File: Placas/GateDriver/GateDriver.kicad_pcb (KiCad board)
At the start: 2 copper layers, 71 x 41 mm, 30 parts, among them J1 Conn_02x04_Odd_Even, J2 Conn_02x04_Odd_Even, Q1 BD135, Q2 BD136, U1 74HC14, U2 LM7815_TO220, U3 HCPL-3120

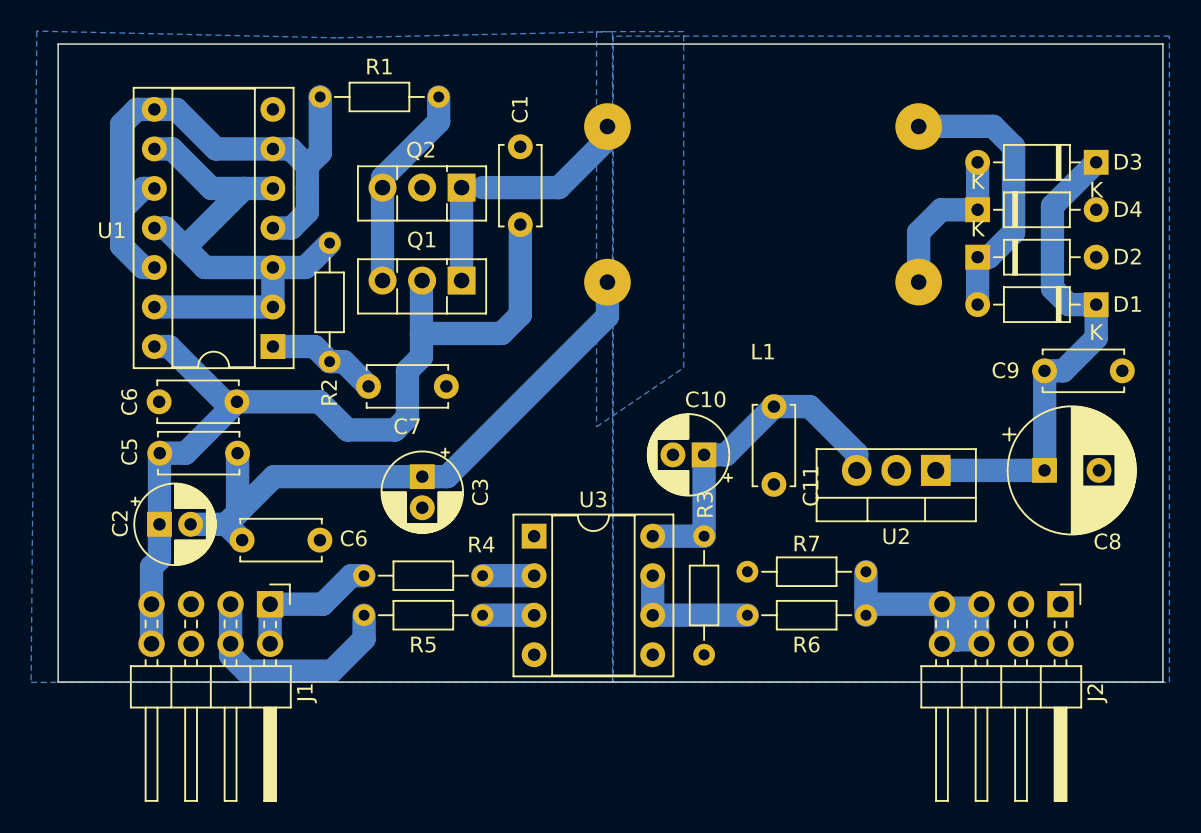
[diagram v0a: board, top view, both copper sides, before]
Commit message: Working
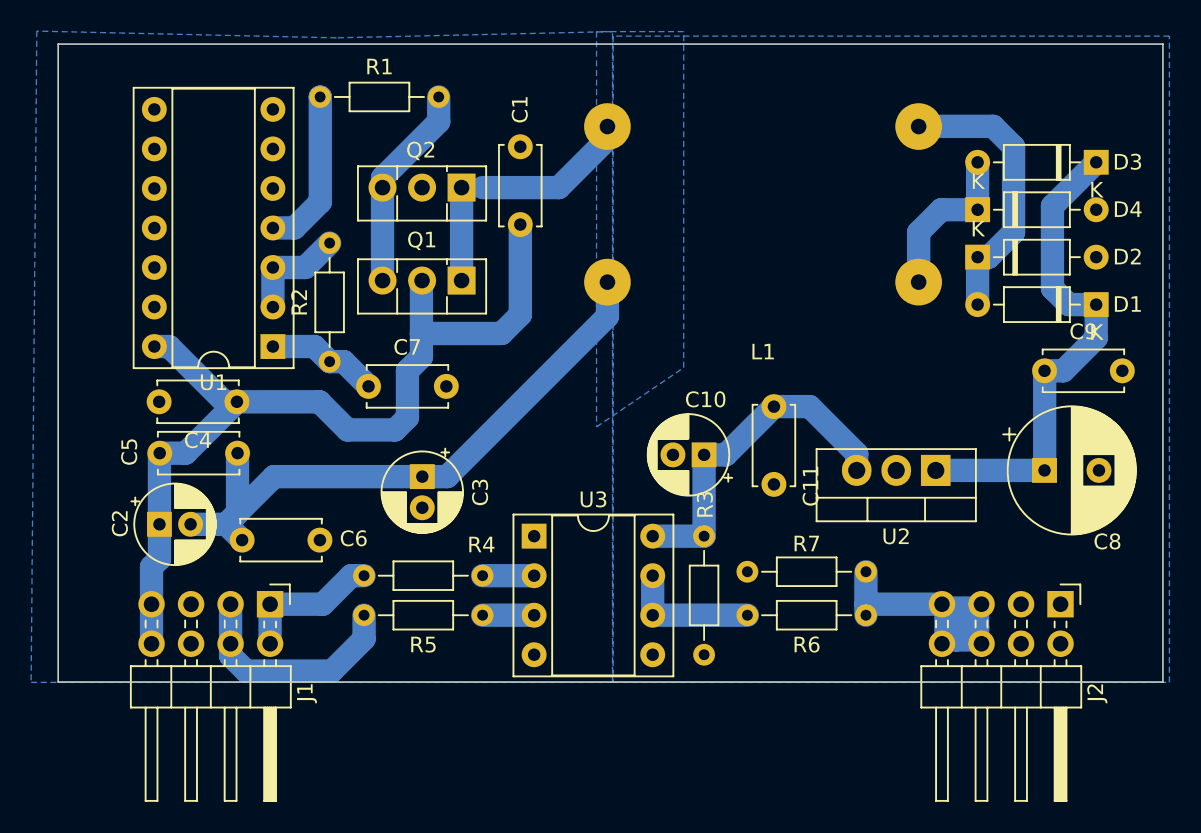
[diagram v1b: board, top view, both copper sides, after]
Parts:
- removed the C6 at (33.5, 47.0)
- added C4: 100n, Capacitor_THT:C_Disc_D5.0mm_W2.5mm_P5.00mm, F.Cu at (33.5, 47.0)
- R1: value 4.7k -> 1k
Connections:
- U1 pad 10: Oscilador -> (no net)
- U1 pad 11: Net-(R2-Pad2) -> (no net)
- U1 pad 12: Oscilador -> (no net)
- U1 pad 13: Net-(R2-Pad2) -> (no net)
- U1 pad 5: Net-(R2-Pad2) -> (no net)
- U1 pad 6: Oscilador -> (no net)
- U1 pad 8: Oscilador -> (no net)
- U1 pad 9: Net-(R2-Pad2) -> (no net)
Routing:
- net Net-(R2-Pad2): track 37.2 -> 6.84 mm
- net Oscilador: track 37.4 -> 10.5 mm
